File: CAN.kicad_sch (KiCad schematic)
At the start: 55 parts, among them J4 Connector, USB-TYPE-C-16P, J6 Conn_01x04, U2 TCAN334D, U3 MIE1W0505BGLVH-3R-Z, U4 MP9485GN-Z, U5 ISO7041FDBQ, U6 ADUM3160, U7 LTV-217-B-G

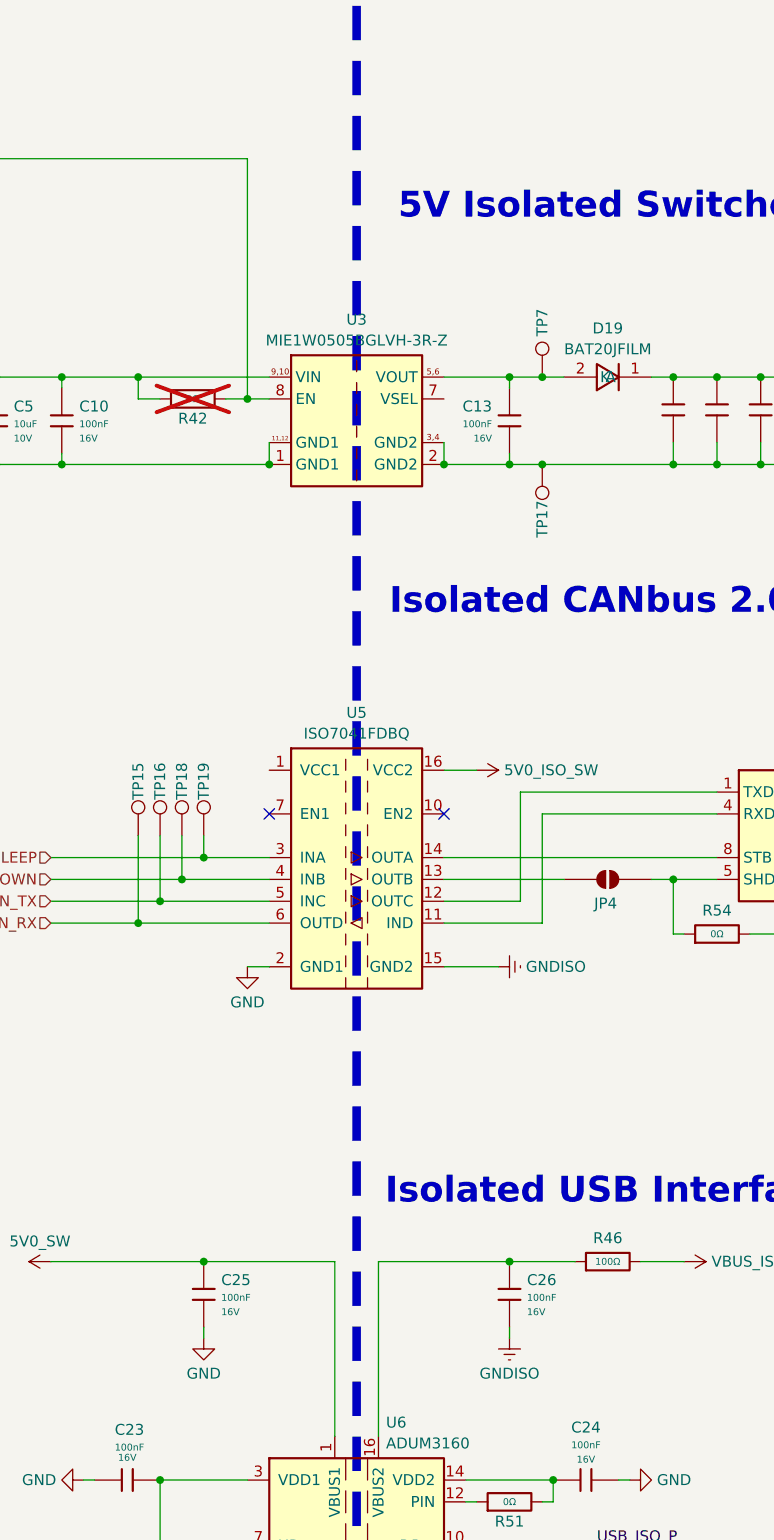
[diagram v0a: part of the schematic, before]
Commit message: Revert "added precharge circuit, filled in placeholder parts"
This reverts commit caa5444a50fe9d2ccb2e95970e40619801e9f697.
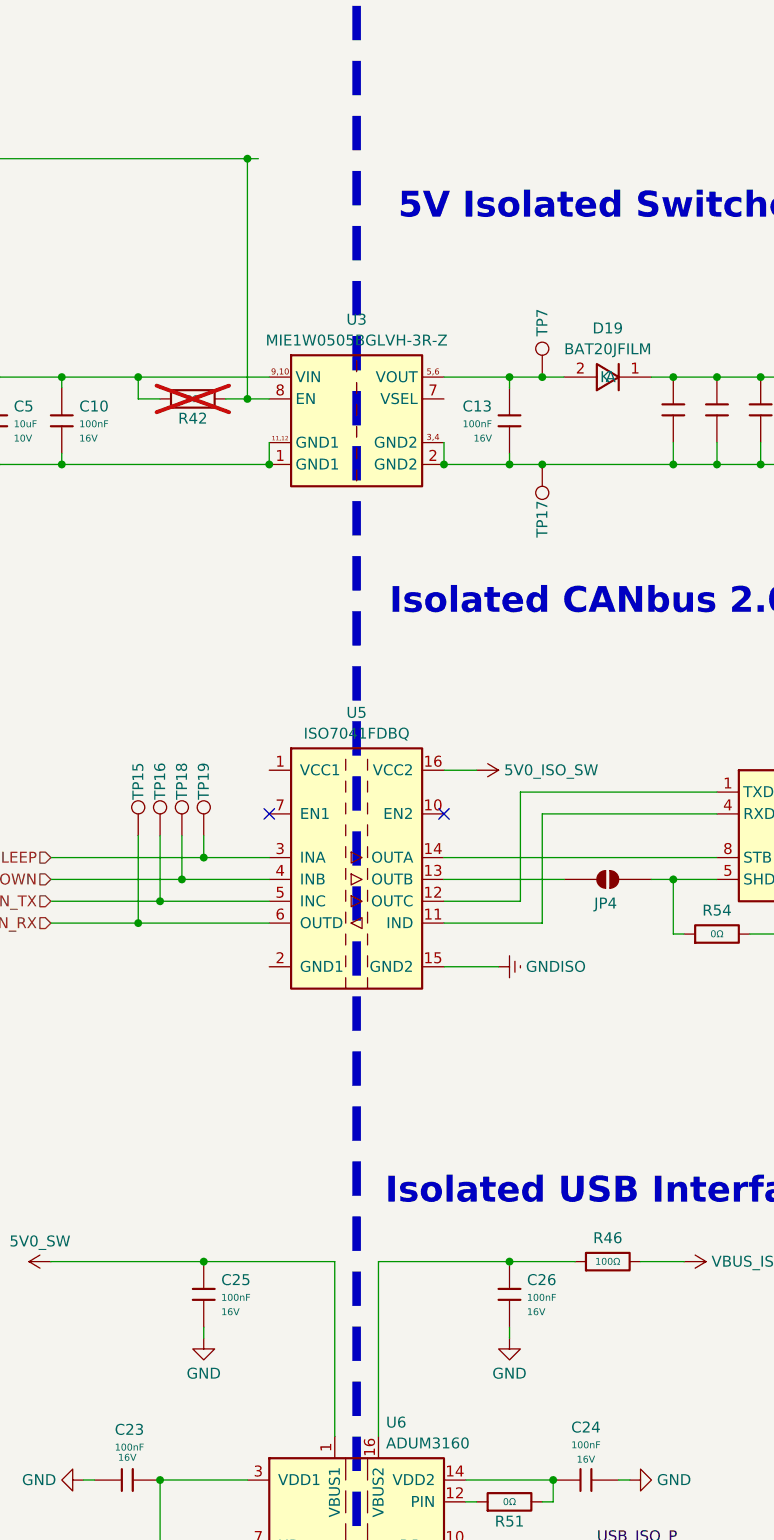
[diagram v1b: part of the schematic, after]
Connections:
- net GND: now also C26.2; no longer U5.2 (GND1), U5.8 (GND1)
- net GNDISO: no longer C26.2
- new net: U5.2 (GND1), U5.8 (GND1)
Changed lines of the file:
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@@
 	)
 	(junction
+		(at 231.14 40.64)
+		(diameter 0)
+		(color 0 0 0 0)
+	)
+	(junction
 		(at 233.68 76.2)
 		(diameter 0)
@@
 	(wire
 		(pts
+			(xy 231.14 40.64) (xy 232.41 40.64)
+		)
+		(stroke
+			(width 0)
+			(type default)
+		)
+	)
+	(wire
+		(pts
 			(xy 231.14 68.58) (xy 228.6 68.58)
 		)
@@
 	(wire
 		(pts
-			(xy 231.14 134.62) (xy 233.68 134.62)
-		)
-		(stroke
-			(width 0)
-			(type default)
-		)
-	)
-	(wire
-		(pts
 			(xy 226.06 176.53) (xy 226.06 177.8)
 		)
@@
 	)
 	(symbol
-		(lib_id "power:Earth")
-		(at 261.62 177.8 0)
-		(unit 1)
-		(body_style 1)
-		(exclude_from_sim no)
-		(in_bom yes)
-		(on_board yes)
-		(in_pos_files yes)
-		(dnp no)
-		(fields_autoplaced yes)
-		(property "Reference" "#PWR051"
-			(at 261.62 184.15 0)
-			(hide yes)
-			(show_name no)
-			(do_not_autoplace no)
-			(effects
-				(font
-					(size 1.27 1.27)
-				)
-			)
-		)
-		(property "Value" "GNDISO"
-			(at 261.62 181.9331 0)
-			(show_name no)
-			(do_not_autoplace no)
-			(effects
-				(font
-					(size 1.27 1.27)
-				)
-			)
-		)
-		(property "Footprint" ""
-			(at 261.62 177.8 0)
-			(hide yes)
-			(show_name no)
-			(do_not_autoplace no)
-			(effects
-				(font
-					(size 1.27 1.27)
-				)
-			)
-		)
-		(property "Datasheet" ""
-			(at 261.62 177.8 0)
-			(hide yes)
-			(show_name no)
-			(do_not_autoplace no)
-			(effects
-				(font
-					(size 1.27 1.27)
-				)
-			)
-		)
-		(property "Description" "Power symbol creates a global label with name \"GNDISO\""
-			(at 261.62 177.8 0)
-			(hide yes)
-			(show_name no)
-			(do_not_autoplace no)
-			(effects
-				(font
-					(size 1.27 1.27)
-				)
-			)
-		)
-		(pin "1"
-		)
-		(instances
-			(project "battery-node"
-				(path "/0531bb65-44fe-462a-8fbf-92fb22c9abe0/a0e287d3-b915-410a-86a7-dfb59e4205a2"
-					(reference "#PWR051")
-					(unit 1)
-				)
-			)
-		)
-	)
-	(symbol
 		(lib_id "PCM_JLCPCB-Resistors:0402,0Ω")
 		(at 257.81 214.63 0)
@@
 	)
 	(symbol
+		(lib_id "power:GND")
+		(at 261.62 177.8 0)
+		(unit 1)
+		(body_style 1)
+		(exclude_from_sim no)
+		(in_bom yes)
+		(on_board yes)
+		(in_pos_files yes)
+		(dnp no)
+		(fields_autoplaced yes)
+		(property "Reference" "#PWR051"
+			(at 261.62 184.15 0)
+			(hide yes)
+			(show_name no)
+			(do_not_autoplace no)
+			(effects
+				(font
+					(size 1.27 1.27)
+				)
+			)
+		)
+		(property "Value" "GND"
+			(at 261.62 181.9331 0)
+			(show_name no)
+			(do_not_autoplace no)
+			(effects
+				(font
+					(size 1.27 1.27)
+				)
+			)
+		)
+		(property "Footprint" ""
+			(at 261.62 177.8 0)
+			(hide yes)
+			(show_name no)
+			(do_not_autoplace no)
+			(effects
+				(font
+					(size 1.27 1.27)
+				)
+			)
+		)
+		(property "Datasheet" ""
+			(at 261.62 177.8 0)
+			(hide yes)
+			(show_name no)
+			(do_not_autoplace no)
+			(effects
+				(font
+					(size 1.27 1.27)
+				)
+			)
+		)
+		(property "Description" "Power symbol creates a global label with name \"GND\" , ground"
+			(at 261.62 177.8 0)
+			(hide yes)
+			(show_name no)
+			(do_not_autoplace no)
+			(effects
+				(font
+					(size 1.27 1.27)
+				)
+			)
+		)
+		(pin "1"
+		)
+		(instances
+			(project "battery-node"
+				(path "/0531bb65-44fe-462a-8fbf-92fb22c9abe0/a0e287d3-b915-410a-86a7-dfb59e4205a2"
+					(reference "#PWR051")
+					(unit 1)
+				)
+			)
+		)
+	)
+	(symbol
 		(lib_id "power:+3V3")
 		(at 208.28 168.91 90)
@@
 					(unit 1)
 				)
-			)
-		)
-	)
-	(symbol
-		(lib_id "power:GND")
-		(at 231.14 134.62 0)
-		(unit 1)
-		(body_style 1)
-		(exclude_from_sim no)
-		(in_bom yes)
-		(on_board yes)
-		(in_pos_files yes)
-		(dnp no)
-		(fields_autoplaced yes)
-		(property "Reference" "#PWR061"
-			(at 231.14 140.97 0)
-			(hide yes)
-			(show_name no)
-			(do_not_autoplace no)
-			(effects
-				(font
-					(size 1.27 1.27)
-				)
-			)
-		)
-		(property "Value" "GND"
-			(at 231.14 138.7531 0)
-			(show_name no)
-			(do_not_autoplace no)
-			(effects
-				(font
-					(size 1.27 1.27)
-				)
-			)
-		)
-		(property "Footprint" ""
-			(at 231.14 134.62 0)
-			(hide yes)
-			(show_name no)
-			(do_not_autoplace no)
-			(effects
-				(font
-					(size 1.27 1.27)
-				)
-			)
-		)
-		(property "Datasheet" ""
-			(at 231.14 134.62 0)
-			(hide yes)
-			(show_name no)
-			(do_not_autoplace no)
-			(effects
-				(font
-					(size 1.27 1.27)
-				)
-			)
-		)
-		(property "Description" "Power symbol creates a global label with name \"GND\" , ground"
-			(at 231.14 134.62 0)
-			(hide yes)
-			(show_name no)
-			(do_not_autoplace no)
-			(effects
-				(font
-					(size 1.27 1.27)
-				)
-			)
-		)
-		(pin "1"
-		)
-		(instances
-			(project "battery-node"
-				(path "/0531bb65-44fe-462a-8fbf-92fb22c9abe0/a0e287d3-b915-410a-86a7-dfb59e4205a2"
-					(reference "#PWR061")
-					(unit 1)
-				)
